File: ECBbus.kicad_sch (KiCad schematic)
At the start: 10 parts, among them J1 IRQ Selection, J10 Bus_ISA_8bit, J2 IRQ Selection, J3 Bus_ISA_8bit, J4 Bus_ISA_8bit, J5 IRQ Selection, J6 Bus_ISA_8bit, J7 IRQ Selection, J8 Bus_ISA_8bit, J9 IRQ Selection

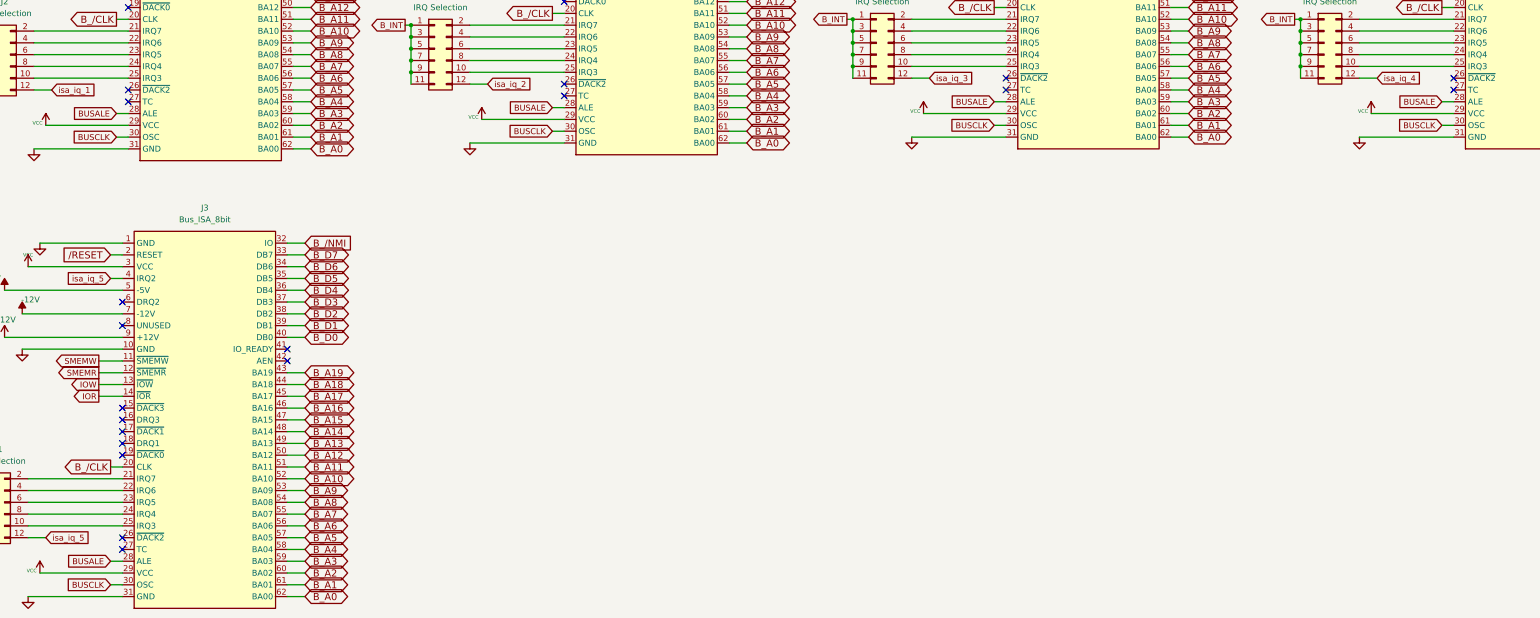
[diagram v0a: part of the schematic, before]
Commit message: V1.1
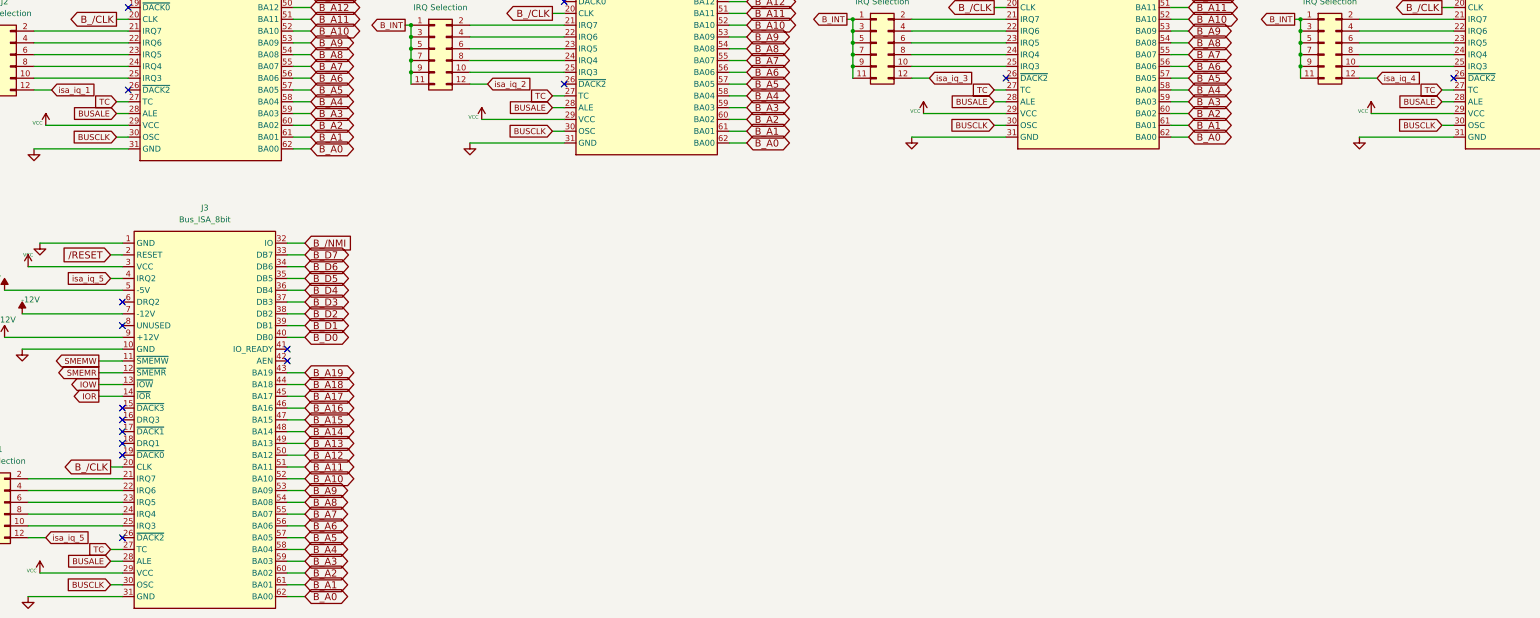
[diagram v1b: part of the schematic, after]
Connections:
- net TC: now reaches J3.27 (TC)
- net TC: now also J10.27 (TC), J4.27 (TC), J6.27 (TC), J8.27 (TC)
- no-connect marks 55 -> 50
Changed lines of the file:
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@@
 	)
 	(no_connect
-		(at 64.77 91.44)
-	)
-	(no_connect
 		(at 63.5 165.1)
 	)
@@
 	)
 	(no_connect
-		(at 350.52 88.9)
-	)
-	(no_connect
 		(at 64.77 43.18)
 	)
@@
 	)
 	(no_connect
-		(at 158.75 90.17)
-	)
-	(no_connect
 		(at 350.52 58.42)
 	)
@@
 	)
 	(no_connect
-		(at 63.5 187.96)
-	)
-	(no_connect
-		(at 254 88.9)
-	)
-	(no_connect
 		(at 100.33 48.26)
 	)
@@
 	(wire
 		(pts
+			(xy 62.23 91.44) (xy 64.77 91.44)
+		)
+		(stroke
+			(width 0)
+			(type default)
+		)
+	)
+	(wire
+		(pts
 			(xy 99.06 167.64) (xy 102.87 167.64)
 		)
@@
 	(wire
 		(pts
+			(xy 251.46 88.9) (xy 254 88.9)
+		)
+		(stroke
+			(width 0)
+			(type default)
+		)
+	)
+	(wire
+		(pts
 			(xy 289.56 99.06) (xy 293.37 99.06)
 		)
@@
 	(wire
 		(pts
+			(xy 156.21 90.17) (xy 158.75 90.17)
+		)
+		(stroke
+			(width 0)
+			(type default)
+		)
+	)
+	(wire
+		(pts
 			(xy 43.18 182.88) (xy 63.5 182.88)
 		)
@@
 	(wire
 		(pts
+			(xy 60.96 187.96) (xy 63.5 187.96)
+		)
+		(stroke
+			(width 0)
+			(type default)
+		)
+	)
+	(wire
+		(pts
 			(xy 330.2 99.06) (xy 350.52 99.06)
 		)
@@
 	(wire
 		(pts
+			(xy 347.98 88.9) (xy 350.52 88.9)
+		)
+		(stroke
+			(width 0)
+			(type default)
+		)
+	)
+	(wire
+		(pts
 			(xy 60.96 170.18) (xy 63.5 170.18)
 		)
@@
 		)
 	)
+	(global_label "TC"
+		(shape input)
+		(at 156.21 90.17 180)
+		(fields_autoplaced yes)
+		(effects
+			(font
+				(size 1.27 1.27)
+			)
+			(justify right)
+		)
+		(property "Intersheetrefs" "${INTERSHEET_REFS}"
+			(at 151.6414 90.17 0)
+			(effects
+				(font
+					(size 1.27 1.27)
+				)
+				(justify right)
+				(hide yes)
+			)
+		)
+	)
 	(global_label "B_D3"
 		(shape bidirectional)
@@
 		)
 	)
+	(global_label "TC"
+		(shape input)
+		(at 251.46 88.9 180)
+		(fields_autoplaced yes)
+		(effects
+			(font
+				(size 1.27 1.27)
+			)
+			(justify right)
+		)
+		(property "Intersheetrefs" "${INTERSHEET_REFS}"
+			(at 246.8914 88.9 0)
+			(effects
+				(font
+					(size 1.27 1.27)
+				)
+				(justify right)
+				(hide yes)
+			)
+		)
+	)
 	(global_label "B_A6"
 		(shape bidirectional)
@@
 		)
 	)
+	(global_label "TC"
+		(shape input)
+		(at 60.96 187.96 180)
+		(fields_autoplaced yes)
+		(effects
+			(font
+				(size 1.27 1.27)
+			)
+			(justify right)
+		)
+		(property "Intersheetrefs" "${INTERSHEET_REFS}"
+			(at 56.3914 187.96 0)
+			(effects
+				(font
+					(size 1.27 1.27)
+				)
+				(justify right)
+				(hide yes)
+			)
+		)
+	)
 	(global_label "B_A15"
 		(shape tri_state)
@@
 		)
 	)
+	(global_label "TC"
+		(shape input)
+		(at 347.98 88.9 180)
+		(fields_autoplaced yes)
+		(effects
+			(font
+				(size 1.27 1.27)
+			)
+			(justify right)
+		)
+		(property "Intersheetrefs" "${INTERSHEET_REFS}"
+			(at 343.4114 88.9 0)
+			(effects
+				(font
+					(size 1.27 1.27)
+				)
+				(justify right)
+				(hide yes)
+			)
+		)
+	)
 	(global_label "B_A0"
 		(shape bidirectional)
@@
 				(hide yes)
 			)
+		)
+	)
+	(global_label "TC"
+		(shape input)
+		(at 62.23 91.44 180)
+		(fields_autoplaced yes)
+		(effects
+			(font
+				(size 1.27 1.27)
+			)
+			(justify right)
+		)
+		(property "Intersheetrefs" "${INTERSHEET_REFS}"
+			(at 57.6614 91.44 0)
+			(effects
+				(font
+					(size 1.27 1.27)
+				)
+				(justify right)
+				(hide yes)
+			)
